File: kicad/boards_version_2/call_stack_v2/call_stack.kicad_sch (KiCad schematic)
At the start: 17 parts

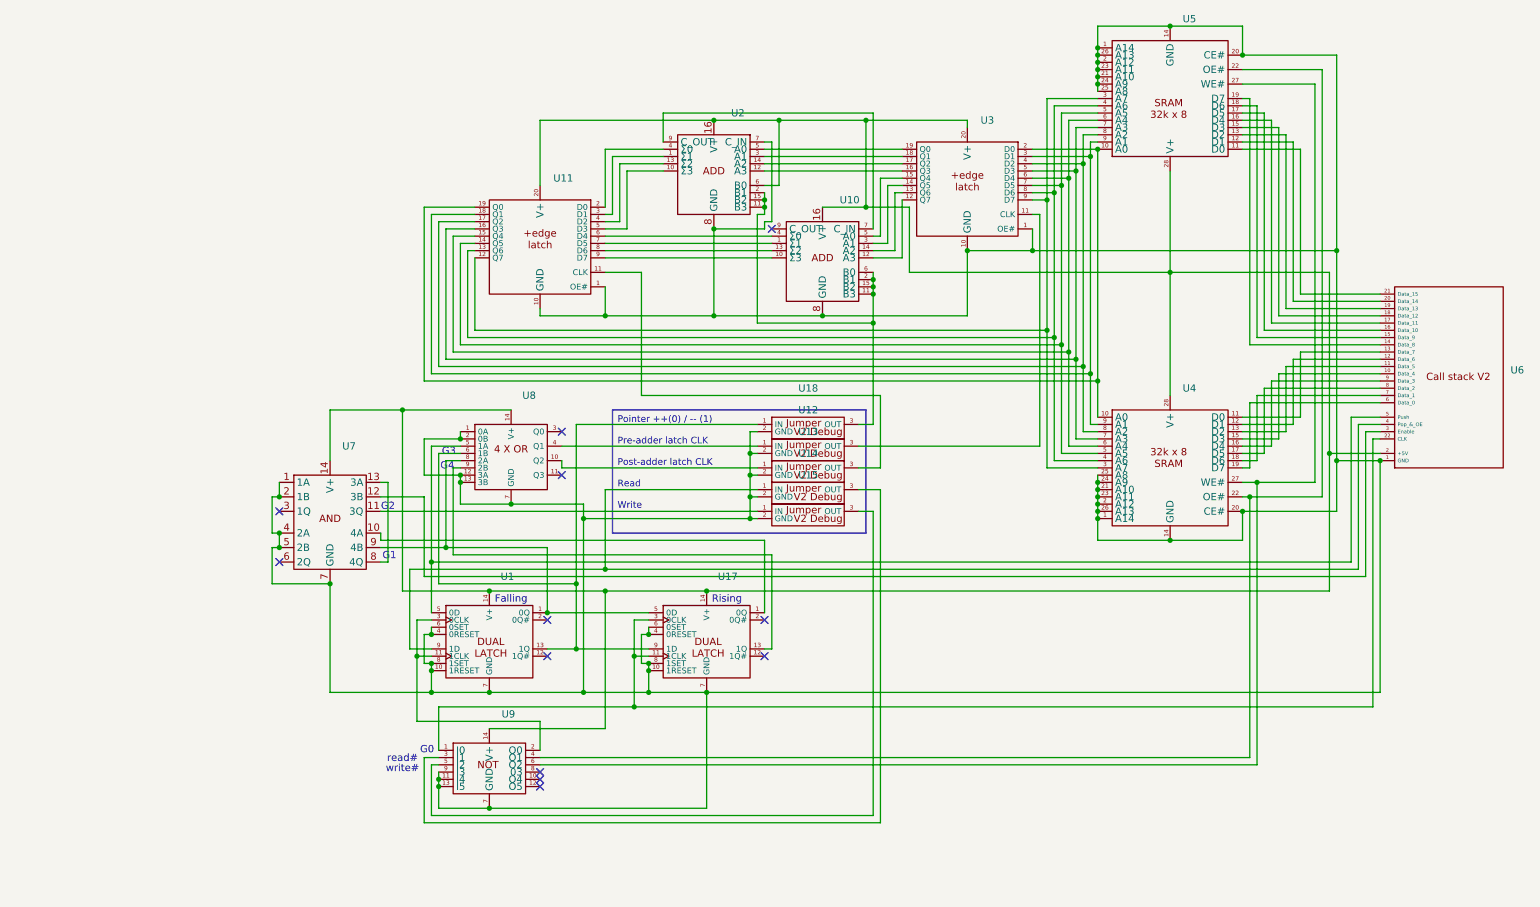
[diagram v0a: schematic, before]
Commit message: Debug figured out and work on ctrl unit main
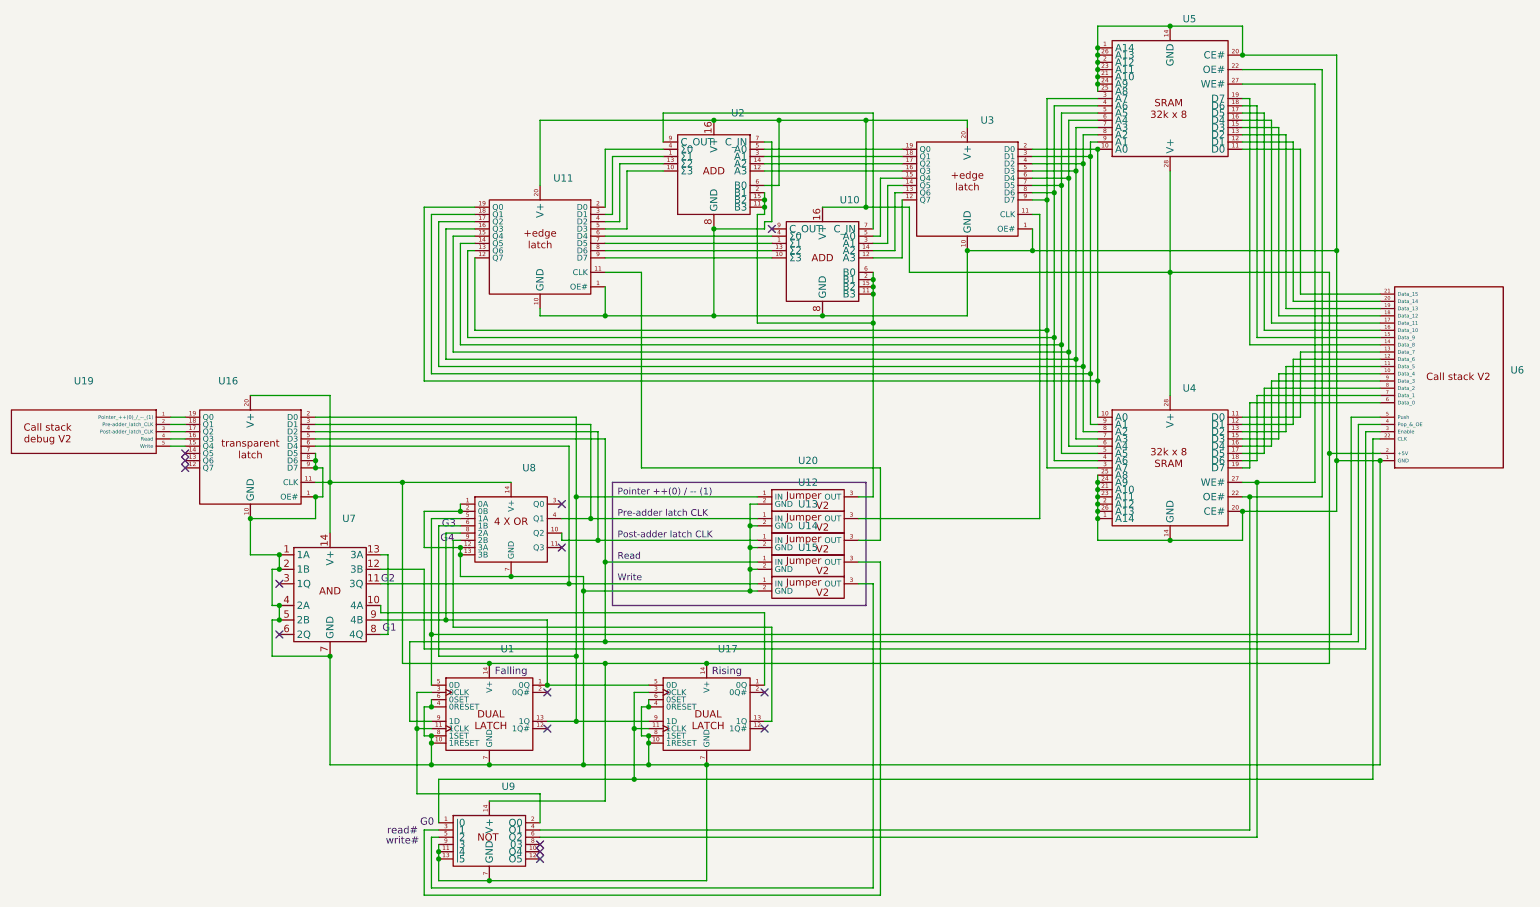
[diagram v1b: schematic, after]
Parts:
- removed U12, U13, U14, U15, U18: ~, custom_footprint_library:jumper_v2_gnd_debug_footprint, symbol custom_symbol_lib:jumper_v2_gnd_debug
- added U12, U13, U14, U15, U20: ~, custom_footprint_library:jumper_v2_gnd_footprint, symbol custom_symbol_lib:jumer_v2_gnd
- added U16: ~, Package_DIP:DIP-20_W7.62mm, symbol custom_symbol_lib:8_bit_transparent_latch
- added U19: ~, Connector_PinHeader_2.54mm:PinHeader_1x05_P2.54mm_Vertical, symbol custom_symbol_lib:debug_v2_call_stack
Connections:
- net at U1.10 (1RESET), U1.4 (0RESET), U1.6 (0SET)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: now also U12.2 (GND), U13.2 (GND), U14.2 (GND), U15.2 (GND), U16.1 (OE#), U16.10 (GND), U16.7 (D5), U16.8 (D6), U16.9 (D7), U20.2 (GND)
- net at U1.14 (V+), U10.16 (V+), U11.20 (V+)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: now also U16.11 (CLK), U16.20 (V+)
- net at U9.3 (I1): now also U14.3 (OUT)
- net at U9.5 (I2): now also U15.3 (OUT)
- net at U1.13 (1Q), U17.9 (1D), U8.6 (1B): now also U16.2 (D0), U20.1 (IN)
- net at U10.11 (B3), U10.15 (B2), U10.2 (B1)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: now also U20.3 (OUT)
- net at U7.11 (3Q): now also U15.1 (IN), U16.6 (D4)
- net at U11.11 (CLK): now also U13.3 (OUT)
- net at U3.11 (CLK): now also U12.3 (OUT)
- net at U8.10 (Q2): now also U13.1 (IN), U16.4 (D2)
- net at U1.9 (1D), U6.4 (Pop_&_OE): now also U14.1 (IN), U16.5 (D3)
- net at U8.4 (Q1): now also U12.1 (IN), U16.3 (D1)
- new net: U16.19 (Q0), U19.1 (Pointer_++(0)_/_--_(1))
- new net: U16.18 (Q1), U19.2 (Pre-adder_latch_CLK)
- new net: U16.17 (Q2), U19.3 (Post-adder_latch_CLK)
- new net: U16.16 (Q3), U19.4 (Read)
- new net: U16.15 (Q4), U19.5 (Write)
- no-connect marks 12 -> 15
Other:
- moved on the sheet: U1, U17, U7, U8, U9
